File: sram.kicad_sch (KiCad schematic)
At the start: 25 parts, among them J1 Cache_slot, M1 UM61256AS, M2 UM61256AS, M3 UM61256AS, M4 UM61256AS, M5 UM61256AS, M6 UM61256AS, M7 UM61256AS, M8 UM61256AS, U1 74HCT244, U2 74HCT244

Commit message: 99% done, ERC DRC 0 errors 0 warnings
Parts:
- CB1, CB2, CB3, CB4: value C -> 1uF 16V
- CT1, CT2, CT3: value C_Polarized -> 10uF 16V
- J1: footprint UM61256AS:Cache slot -> footprints:Cache slot; symbol New_Library:Cache_slot -> cache_slot:Cache_slot
- M1, M2, M3, M4, M5, M6, M7, M8: footprint UM61256AS:SOJ28_18P54X7P75_ISI -> footprints:SOJ28_18P54X7P75_ISI; symbol Memory_RAM:HM62256BLP -> um61256as_slim:UM61256AS_slim
- MD1: footprint UM61256AS:SOJ28_18P54X7P75_ISI -> footprints:SOJ28_18P54X7P75_ISI; symbol Memory_RAM:HM62256BLP -> um61256as_slim:UM61256AS_slim; Field4 TAG -> (none)
- U1, U2: value 74HCT244 -> 74F244
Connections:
- net +5V: now also J1.b11, J1.b15, J1.b19, J1.b31, J1.b39, J1.b43, J1.b52, J1.b7; no longer J1.B14, J1.B18, J1.B26, J1.B38, J1.B42, J1.B46, J1.B50, J1.B7
- net Bank0_CS: now also J1.a34, J1.a35, J1.a36, J1.a38; no longer J1.A2
- net Bank0_OE: now also J1.b58; no longer J1.B1
- net Bank1_CS: now also J1.a28, J1.a30, J1.a31, J1.a32; no longer J1.A3, R6.1
- net Bank1_OE: now also J1.b57; no longer J1.B2
- net Byte_WE0: now also J1.b44, J1.b51; no longer J1.B13, J1.B8
- net Byte_WE1: now also J1.b45, J1.b53; no longer J1.B12, J1.B6
- net Byte_WE2: now also J1.b49, J1.b54; no longer J1.B10, J1.B5
- net Byte_WE3: now also J1.b50, J1.b55; no longer J1.B4, J1.B9
- net CPU_A10: now also J1.a14; no longer J1.A43
- net CPU_A11: now also J1.a12; no longer J1.A45
- net CPU_A12: now also J1.a11; no longer J1.A46
- net CPU_A13: now also J1.a10; no longer J1.A47
- net CPU_A14: now also J1.a8; no longer J1.A49
- net CPU_A15: now also J1.a7; no longer J1.A50
- net CPU_A16: now also J1.a6; no longer J1.A51
- net CPU_A17: now also J1.a4; no longer J1.A53
- net CPU_A4: now also J1.a22; no longer J1.A35
- net CPU_A5: now also J1.a20; no longer J1.A37
- net CPU_A6: now also J1.a19; no longer J1.A38
- net CPU_A7: now also J1.a18; no longer J1.A39
- net CPU_A8: now also J1.a16; no longer J1.A41
- net CPU_A9: now also J1.a15; no longer J1.A42
- net CPU_D0: now also J1.b1; no longer J1.B56
- net CPU_D1: now also J1.b2; no longer J1.B55
- net CPU_D10: now also J1.b14; no longer J1.B43
- net CPU_D11: now also J1.b16; no longer J1.B41
- net CPU_D12: now also J1.b17; no longer J1.B40
- net CPU_D13: now also J1.b18; no longer J1.B39
- net CPU_D14: now also J1.b20; no longer J1.B37
- net CPU_D15: now also J1.b21; no longer J1.B36
- net CPU_D16: now also J1.b22; no longer J1.B35
- net CPU_D17: now also J1.b24; no longer J1.B33
- net CPU_D18: now also J1.b25; no longer J1.B32
- net CPU_D19: now also J1.b26; no longer J1.B31
- net CPU_D2: now also J1.b4; no longer J1.B53
- net CPU_D20: now also J1.b28; no longer J1.B29
- net CPU_D21: now also J1.b29; no longer J1.B28
- net CPU_D22: now also J1.b30; no longer J1.B27
- net CPU_D23: now also J1.b32; no longer J1.B25
- net CPU_D24: now also J1.b33; no longer J1.B24
- net CPU_D25: now also J1.b34; no longer J1.B23
- net CPU_D26: now also J1.b36; no longer J1.B21
- net CPU_D27: now also J1.b37; no longer J1.B20
- net CPU_D28: now also J1.b38; no longer J1.B19
- net CPU_D29: now also J1.b40; no longer J1.B17
- net CPU_D3: now also J1.b5; no longer J1.B52
- net CPU_D30: now also J1.b41; no longer J1.B16
- net CPU_D31: now also J1.b42; no longer J1.B15
- net CPU_D4: now also J1.b6; no longer J1.B51
- net CPU_D5: now also J1.b8; no longer J1.B49
- net CPU_D6: now also J1.b9; no longer J1.B48
- net CPU_D7: now also J1.b10; no longer J1.B47
- net CPU_D8: now also J1.b12; no longer J1.B45
- net CPU_D9: now also J1.b13; no longer J1.B44
- net GND: now also J1.a1, J1.a13, J1.a17, J1.a21, J1.a25, J1.a29, J1.a33, J1.a37, J1.a41, J1.a45, J1.a5, J1.a50, J1.a54, J1.a9, J1.b23, J1.b27, J1.b3, J1.b35, J1.b48, J1.b56, U1.2 (1A0); no longer J1.A12, J1.A16, J1.A20, J1.A24, J1.A28, J1.A32, J1.A36, J1.A40, J1.A44, J1.A48, J1.A5, J1.A52, J1.A56, J1.A9, J1.B11, J1.B22, J1.B3, J1.B30, J1.B34, J1.B54
- net TAG_Q0: now also J1.a39; no longer J1.A18
- net TAG_Q1: now also J1.a40; no longer J1.A17
- net TAG_Q2: now also J1.a42; no longer J1.A15
- net TAG_Q3: now also J1.a43; no longer J1.A14
- net TAG_Q4: now also J1.a44; no longer J1.A13
- net TAG_Q5: now also J1.a48; no longer J1.A11
- net TAG_Q6: now also J1.a49; no longer J1.A10
- net TAG_Q7: now also J1.a51; no longer J1.A8
- net TAG_WE: now also J1.a55; no longer J1.A4
- removed net CPU_A4_SR: M1.10 (A0), M2.10 (A0), M3.10 (A0), M4.10 (A0), M5.10 (A0), M6.10 (A0), M7.10 (A0), M8.10 (A0), U1.18 (1Y0)
- removed net under_U1_2: J1.A25, J1.A26, J1.A27, J1.A29
- removed net under_U1_3: J1.A19, J1.A21, J1.A22, J1.A23
- new net Bank0_A0: J1.a57, M1.10 (A0), M2.10 (A0), M3.10 (A0), M4.10 (A0)
- new net Bank1_A0: J1.a56, M5.10 (A0), M6.10 (A0), M7.10 (A0), M8.10 (A0), R6.1
- no-connect marks 10 -> 2
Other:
- note removed: "?"
- note removed: "Bank0_CS??"
- note removed: "Bank1_CS??"
- note removed: "Cache size: | short: 256K (2 banks)|R1 R3 R5 128K (1 bank) |R2 R3 R6 64KB (2 banks)|R2 R4 ??"
- company: (none) -> Rasz_pl
- title: (none) -> Cache slot for FIC 486-GAC2
- moved on the sheet: CB1, CB2, CB3, CB4, CT1, CT2, CT3, M1, M2, M3, M4, M5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

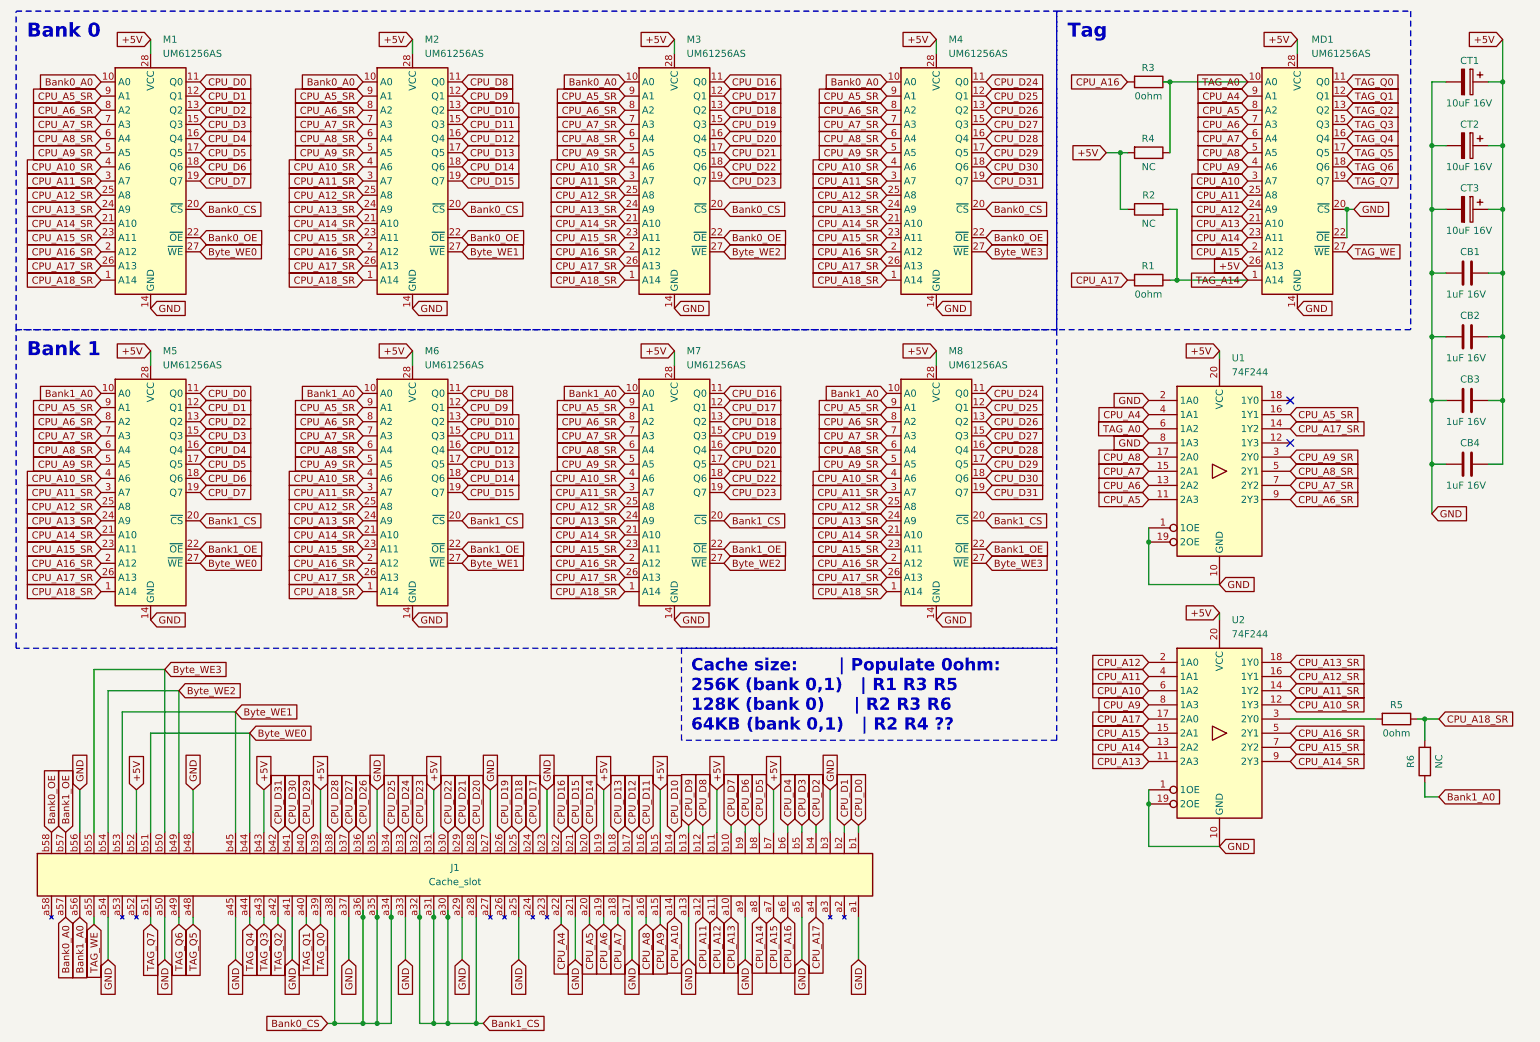
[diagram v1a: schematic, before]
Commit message: config description correction
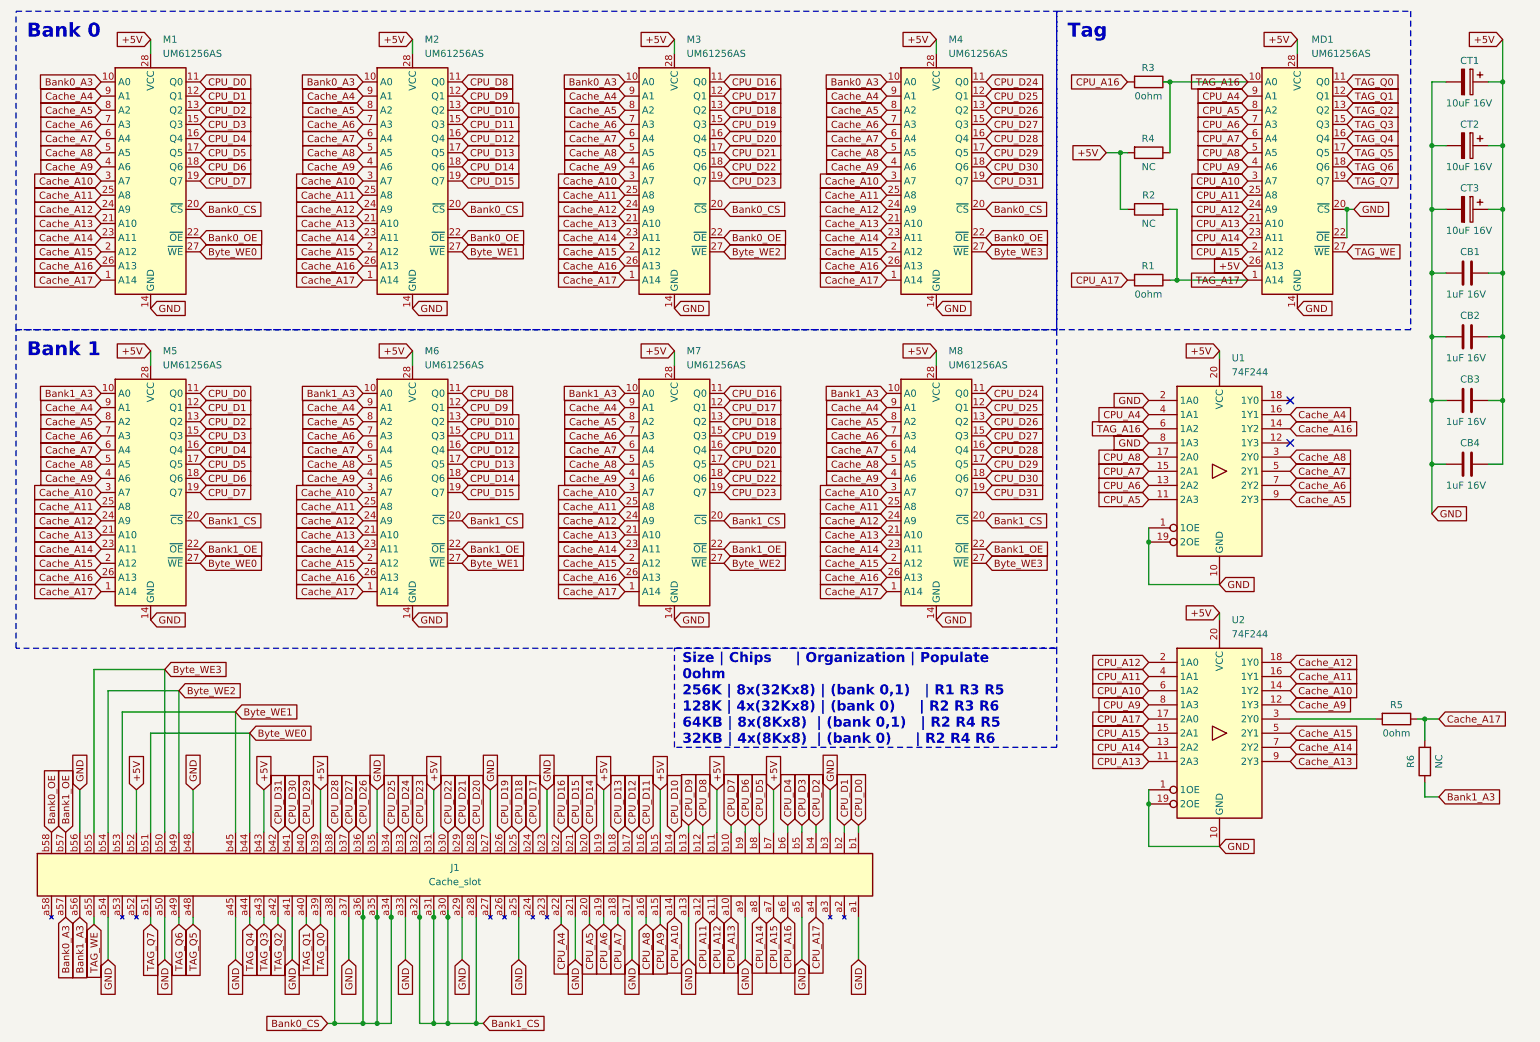
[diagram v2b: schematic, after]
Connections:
- net Bank0_A0 renamed Bank0_A3
- net Bank1_A0 renamed Bank1_A3
- net CPU_A10_SR renamed Cache_A9
- net CPU_A11_SR renamed Cache_A10
- net CPU_A12_SR renamed Cache_A11
- net CPU_A13_SR renamed Cache_A12
- net CPU_A14_SR renamed Cache_A13
- net CPU_A15_SR renamed Cache_A14
- net CPU_A16_SR renamed Cache_A15
- net CPU_A17_SR renamed Cache_A16
- net CPU_A18_SR renamed Cache_A17
- net CPU_A5_SR renamed Cache_A4
- net CPU_A6_SR renamed Cache_A5
- net CPU_A7_SR renamed Cache_A6
- net CPU_A8_SR renamed Cache_A7
- net CPU_A9_SR renamed Cache_A8
- net TAG_A0 renamed TAG_A16
- net TAG_A14 renamed TAG_A17
